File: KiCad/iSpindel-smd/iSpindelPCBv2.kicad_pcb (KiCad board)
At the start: 2 copper layers, 46 x 25 mm, 20 parts, among them J1 PROG, J2 PROG_con, SW1 SW_DPDT_x2, U1 MIC5219-3.3, U2 GY-521, U3 TP4056-shield-6PIN, U4 DS18B20, U5 LoRa_Ra-02, U6 ESP-07S

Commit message: adjust switch and charger
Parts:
- U3: footprint TP4056-shield-6PIN -> KiCadCustomLibs:TP4056-shield-6PIN
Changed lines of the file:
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@@
-(kicad_pcb (version 4) (host pcbnew 4.0.6)
+(kicad_pcb (version 4) (host pcbnew 4.0.7)
   (general
     (links 51)
     (no_connects 51)
-    (area 124.275 60.05 176.025001 92.938095)
+    (area 125.924999 65.924999 172.075001 91.075001)
     (thickness 1.6)
     (drawings 8)
@@
     (add_net VCC)
   )
-  (module TP4056-shield-6PIN (layer B.Cu)
-    (at 158.5 78.5 180)
-    (fp_text reference U3 (at 0.5 0 180) (layer B.SilkS)
-      (effects (font (size 1 1) (thickness 0.15)) (justify mirror))
-    )
-    (fp_text value TP4056-shield-6PIN (at 0 7 180) (layer B.Fab) hide
-      (effects (font (size 1 1) (thickness 0.15)) (justify mirror))
-    )
-    (fp_line (start -14.5 -4) (end -9.5 -4) (layer B.Fab) (width 0.15))
-    (fp_line (start 13 6) (end 13 -6) (layer B.SilkS) (width 0.15))
-    (fp_line (start 13 6) (end 14.5 6) (layer B.SilkS) (width 0.15))
-    (fp_line (start 14.5 6) (end 14.5 8.5) (layer B.SilkS) (width 0.15))
-    (fp_line (start 14.5 8.5) (end 13.5 8.5) (layer B.SilkS) (width 0.15))
-    (fp_line (start 13 -6) (end 14.5 -6) (layer B.SilkS) (width 0.15))
-    (fp_line (start 14.5 -6) (end 14.5 -8.5) (layer B.SilkS) (width 0.15))
-    (fp_line (start 14.5 -8.5) (end 13.5 -8.5) (layer B.SilkS) (width 0.15))
-    (fp_line (start -9.5 -4) (end -9.5 4) (layer B.Fab) (width 0.15))
-    (fp_line (start -9.5 4) (end -14.5 4) (layer B.Fab) (width 0.15))
-    (fp_line (start -14.5 4) (end -14.5 -4) (layer B.Fab) (width 0.15))
-    (fp_line (start -13.5 -8.5) (end -13.5 8.5) (layer B.SilkS) (width 0.15))
-    (fp_line (start -13.5 8.5) (end 13.5 8.5) (layer B.SilkS) (width 0.15))
-    (fp_line (start 13.5 -8.5) (end -13.5 -8.5) (layer B.SilkS) (width 0.15))
-    (pad 3 thru_hole oval (at 11.1 7 180) (size 3 2) (drill 1) (layers *.Cu *.Mask)
-      (net 20 "Net-(SW1-Pad2)"))
-    (pad 4 thru_hole oval (at 11.1 -7 180) (size 3 2) (drill 1) (layers *.Cu *.Mask)
-      (net 10 "Net-(U3-Pad4)"))
-    (pad 2 thru_hole oval (at -11.5 -7 180) (size 3 2) (drill 1) (layers *.Cu *.Mask)
-      (net 1 GND))
-    (pad 1 thru_hole oval (at -11.5 7 180) (size 3 2) (drill 1) (layers *.Cu *.Mask)
-      (net 11 "Net-(U3-Pad1)"))
-  )
   (module ESP-07S (layer F.Cu)
     (at 136.25 75.5 270)
@@
       (net 17 VCC))
   )
+  (module KiCadCustomLibs:TP4056-shield-6PIN (layer B.Cu)
+    (at 158.5 78.5 180)
+    (fp_text reference U3 (at 0.5 0 180) (layer B.SilkS)
+      (effects (font (size 1 1) (thickness 0.15)) (justify mirror))
+    )
+    (fp_text value TP4056-shield-6PIN (at 0 7 180) (layer B.Fab) hide
+      (effects (font (size 1 1) (thickness 0.15)) (justify mirror))
+    )
+    (fp_line (start -14.5 -4) (end -9.5 -4) (layer B.Fab) (width 0.15))
+    (fp_line (start 13 6) (end 13 -6) (layer B.SilkS) (width 0.15))
+    (fp_line (start 13 6) (end 14.5 6) (layer B.SilkS) (width 0.15))
+    (fp_line (start 14.5 6) (end 14.5 8.5) (layer B.SilkS) (width 0.15))
+    (fp_line (start 14.5 8.5) (end 13.5 8.5) (layer B.SilkS) (width 0.15))
+    (fp_line (start 13 -6) (end 14.5 -6) (layer B.SilkS) (width 0.15))
+    (fp_line (start 14.5 -6) (end 14.5 -8.5) (layer B.SilkS) (width 0.15))
+    (fp_line (start 14.5 -8.5) (end 13.5 -8.5) (layer B.SilkS) (width 0.15))
+    (fp_line (start -9.5 -4) (end -9.5 4) (layer B.Fab) (width 0.15))
+    (fp_line (start -9.5 4) (end -14.5 4) (layer B.Fab) (width 0.15))
+    (fp_line (start -14.5 4) (end -14.5 -4) (layer B.Fab) (width 0.15))
+    (fp_line (start -13.5 -8.5) (end -13.5 8.5) (layer B.SilkS) (width 0.15))
+    (fp_line (start -13.5 8.5) (end 13.5 8.5) (layer B.SilkS) (width 0.15))
+    (fp_line (start 13.5 -8.5) (end -13.5 -8.5) (layer B.SilkS) (width 0.15))
+    (pad 3 thru_hole oval (at 11.1 7 180) (size 3 2) (drill 1) (layers *.Cu *.Mask)
+      (net 20 "Net-(SW1-Pad2)"))
+    (pad 4 thru_hole oval (at 11.1 -7 180) (size 3 2) (drill 1) (layers *.Cu *.Mask)
+      (net 10 "Net-(U3-Pad4)"))
+    (pad 2 thru_hole oval (at -11.5 -7 180) (size 3 2) (drill 1) (layers *.Cu *.Mask)
+      (net 1 GND))
+    (pad 1 thru_hole oval (at -11.5 7 180) (size 3 2) (drill 1) (layers *.Cu *.Mask)
+      (net 11 "Net-(U3-Pad1)"))
+    (model ../../../../../../src/Tennp/Git/KiCadCustomLibs/wrl/TP4056shield.wrl
+      (at (xyz 0 0 0))
+      (scale (xyz 0.395 0.395 0.395))
+      (rotate (xyz 0 0 180))
+    )
+    (model ../../../../../../src/Tennp/Git/KiCadCustomLibs/wrl/Conn_USB-micro-2.0_socket_right-angle.wrl
+      (at (xyz -0.47 0 0.047))
+      (scale (xyz 1 1 1))
+      (rotate (xyz 0 0 0))
+    )
+  )
   (dimension 22.5 (width 0.3) (layer Dwgs.User)

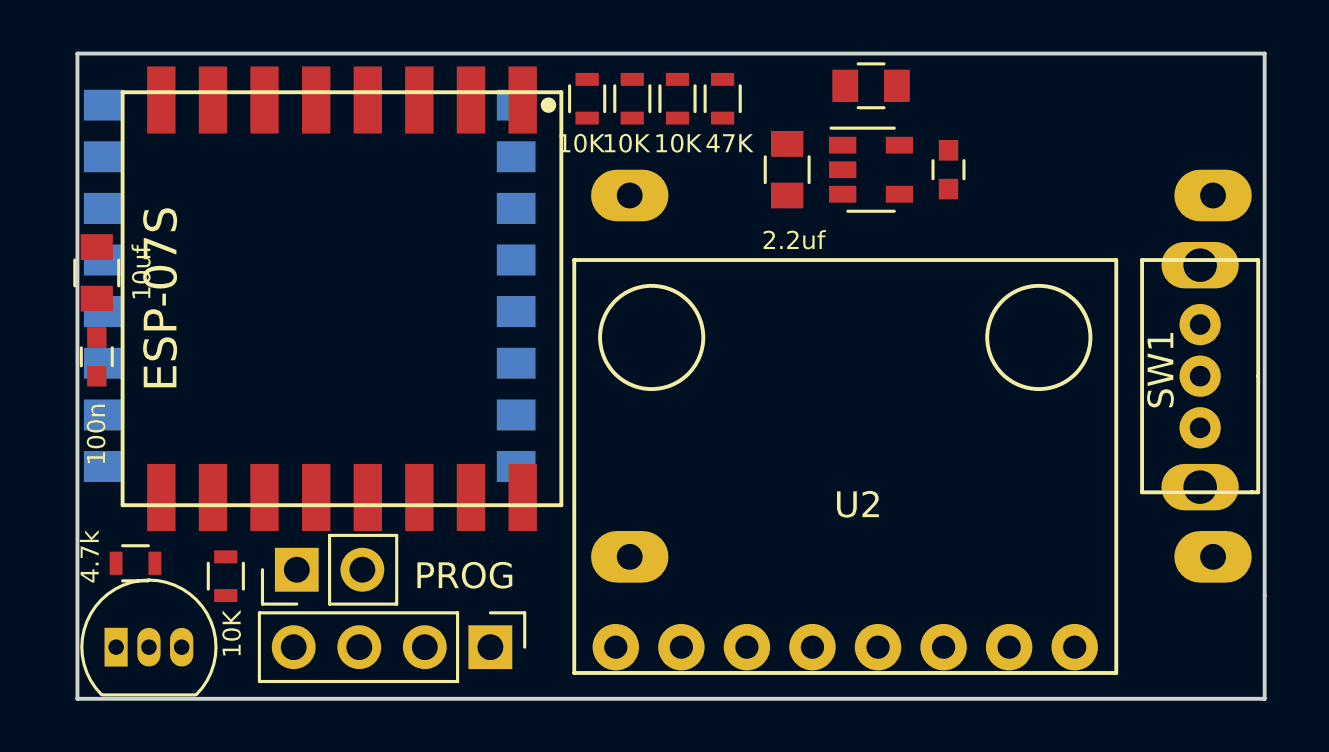
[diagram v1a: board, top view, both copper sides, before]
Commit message: Some work still in progress
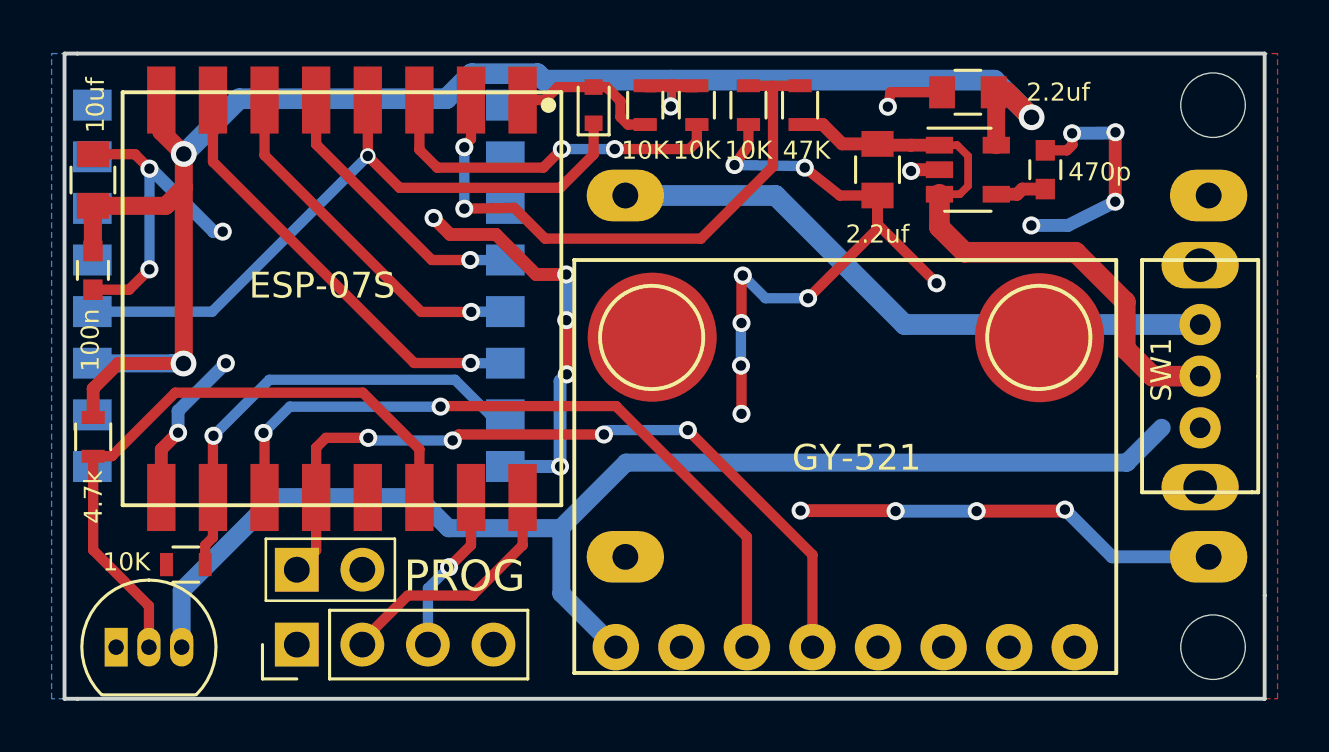
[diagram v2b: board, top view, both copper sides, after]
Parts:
- added D1: Schottky, Diodes_SMD:D_SOD-523, F.Cu at (146.0, 68.0)
- added REF**: MountingHole_3.2mm_M3, Mounting_Holes:MountingHole_3.2mm_M3, F.Cu at (163.3, 77.0)
- added REF**: MountingHole_3.2mm_M3, Mounting_Holes:MountingHole_3.2mm_M3, F.Cu at (148.3, 77.0)
- added REF**: MountingHole_3.2mm_M3, Mounting_Holes:MountingHole_3.2mm_M3, F.Cu at (170.0, 89.0)
- added REF**: MountingHole_3.2mm_M3, Mounting_Holes:MountingHole_3.2mm_M3, F.Cu at (170.0, 68.0)
- SW1: value SW_DPDT_x2 -> SW_SPDT
- moved J2 7.50 mm to (134.5, 88.9), turned to 90 degrees
- moved R2 5.17 mm to (126.6, 80.8), turned to 270 degrees
- moved R4 4.26 mm to (150.0, 68.0)
- moved C3 3.76 mm to (160.5, 67.5)
- moved C2 3.75 mm to (163.5, 70.5)
- moved U1 3.75 mm to (160.5, 70.5)
- moved C5 3.60 mm to (126.6, 70.9)
- moved C1 3.50 mm to (157.0, 70.5), turned to 270 degrees
- moved C4 3.35 mm to (126.6, 74.4)
- moved R1 3.01 mm to (154.0, 68.0)
- moved R3 2.76 mm to (152.0, 68.0), turned to 270 degrees
- moved R6 1.61 mm to (130.2, 85.8), turned to 0 degrees
- moved R5 0.56 mm to (148.0, 68.0)
- moved U5 0.42 mm to (134.6, 75.0)
- moved U3 0.17 mm to (158.3, 78.5)
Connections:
- J2 pad 4: VCC -> /VCC_PROG
- SW1 pad 1: VCC -> /VCC_PROG
- SW1 pad 2: Net-(SW1-Pad2) -> VCC
- U2 pad 5: Net-(U2-Pad5) -> (no net)
- U2 pad 6: Net-(U2-Pad6) -> (no net)
- U2 pad 7: Net-(U2-Pad7) -> (no net)
- U2 pad 8: Net-(U2-Pad8) -> (no net)
- U3 pad 1: Net-(U3-Pad1) -> (no net)
- U3 pad 3: Net-(SW1-Pad2) -> Net-(SW1-Pad3)
- U3 pad 4: Net-(U3-Pad4) -> (no net)
- U5 pad 10: Net-(U5-Pad10) -> (no net)
- U5 pad 11: Net-(U5-Pad11) -> (no net)
- U5 pad 5: Net-(U5-Pad5) -> (no net)
- U5 pad 6: Net-(U5-Pad6) -> (no net)
- U5 pad 7: Net-(U5-Pad7) -> (no net)
- U5 pad 8: Net-(U5-Pad8) -> (no net)
- U6 pad 13: Net-(U6-Pad13) -> (no net)
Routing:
- net GND: track 0.00 -> 89.4 mm, vias 0 -> 28
- net VCC: track 0.00 -> 73.6 mm
- net +3V3: track 0.00 -> 67.5 mm, vias 0 -> 4
- net /SDA: track 0.00 -> 30.6 mm, vias 0 -> 4
- net /SCL: track 0.00 -> 28.0 mm, vias 0 -> 2
- net /RES: track 0.00 -> 25.9 mm, vias 0 -> 1
- net /Temp: track 0.00 -> 24.7 mm
- net Net-(SW1-Pad3): track 0.00 -> 24.5 mm, vias 0 -> 1
- net Net-(R1-Pad2): track 0.00 -> 23.1 mm, vias 0 -> 2
- net /NSS: track 0.00 -> 18.3 mm, vias 0 -> 1
- net /MOSI: track 0.00 -> 17.4 mm, vias 0 -> 1
- net /MISO: track 0.00 -> 14.4 mm, vias 0 -> 1
- net /EN: track 0.00 -> 14.0 mm, vias 0 -> 2
- net /SCK: track 0.00 -> 11.3 mm, vias 0 -> 1
- net Net-(J2-Pad2): track 0.00 -> 9.74 mm
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- added copper zone on B.Cu, net GND
- added copper zone on F.Cu, net GND
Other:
- board size 46 x 25 mm -> 46.5 x 25 mm
- net class Default: trace_width 0.25 -> 0.4; via_dia 0.6 -> 0.7
- net class VCC added: clearance 0.2, trace_width 0.7, via_dia 1, via_drill 0.6
- rule pad_to_mask_clearance: 0.2 -> 0.15
- board text added: "DS18B20"
- board text added: "GND"
- board text added: "LoRa Ra-02"
- board text added: "OUT+"
- board text added: "RX"
- board text added: "TP4056"
- board text added: "TX"
- board text added: "VCC"
- board text added: "short for prog"
- board text added: "www.ispindel.de"
